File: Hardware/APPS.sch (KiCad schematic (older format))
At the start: 20 parts, among them SW1 SW_Push, U1 STM32F103C8Tx, Y1 Crystal 8 MHz

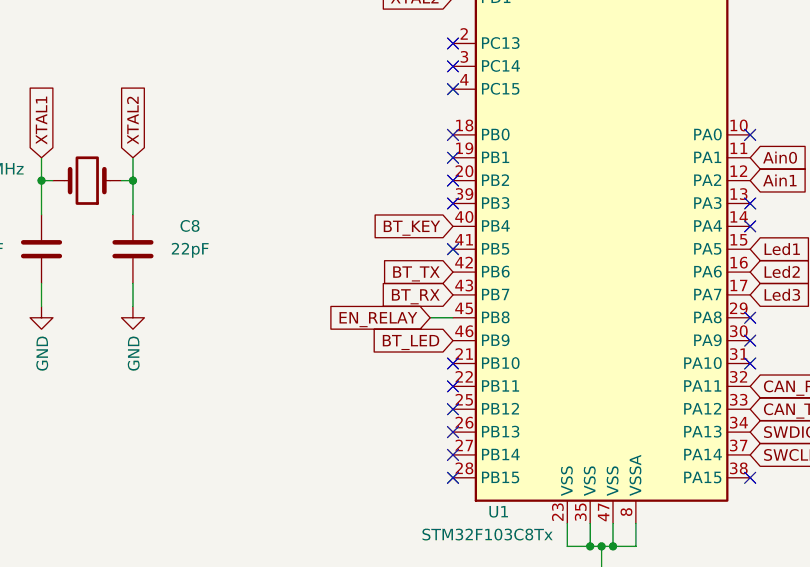
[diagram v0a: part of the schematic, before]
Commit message: Quick fixes
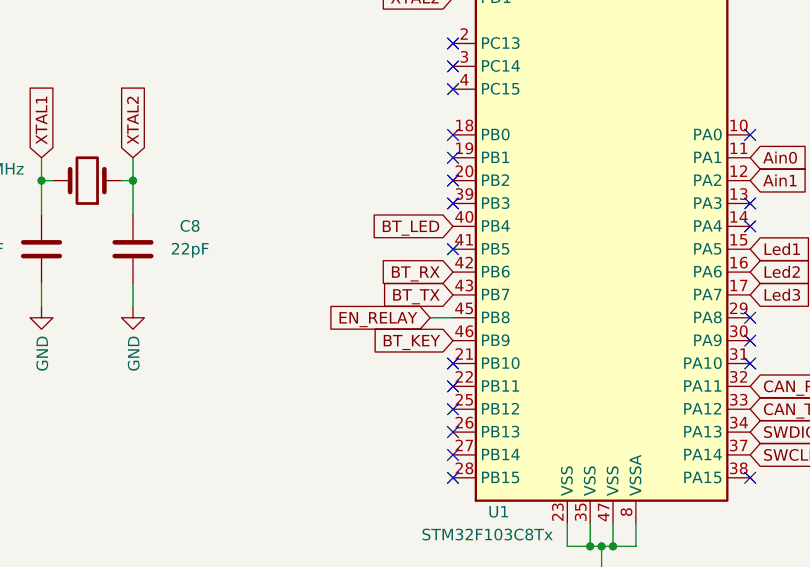
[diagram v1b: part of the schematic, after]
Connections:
- net BT_KEY: now also U1.46 (PB9); no longer U1.40 (PB4)
- net BT_LED: now also U1.40 (PB4); no longer U1.46 (PB9)
- net BT_RX: now also U1.42 (PB6); no longer U1.43 (PB7)
- net BT_TX: now also U1.43 (PB7); no longer U1.42 (PB6)
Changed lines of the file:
@@
 NoConn ~ 4200 4850
 NoConn ~ 4200 4750
-NoConn ~ 4200 4650
-NoConn ~ 4200 4150
 NoConn ~ 5500 4050
 NoConn ~ 5500 3950
@@
 Text Notes 7850 2700 0    50   ~ 0
 Debugging Diodes
-Text GLabel 4200 4350 0    50   Input ~ 0
-BT_RX
-Text GLabel 4200 4250 0    50   Input ~ 0
-BT_TX
 Text GLabel 5500 4150 2    50   Input ~ 0
 Led1
-Text GLabel 4200 4050 0    50   Input ~ 0
-BT_KEY
-Text GLabel 4200 4550 0    50   Input ~ 0
-BT_LED
 NoConn ~ 5500 4550
 NoConn ~ 5500 4650
 Text GLabel 5500 4750 2    50   Input ~ 0
 CAN_RX
+Text GLabel 4200 4550 0    50   Input ~ 0
+BT_KEY
+NoConn ~ 4200 4650
+Text GLabel 4200 4250 0    50   Input ~ 0
+BT_RX
+Text GLabel 4200 4350 0    50   Input ~ 0
+BT_TX
+NoConn ~ 4200 4150
+Text GLabel 4200 4050 0    50   Input ~ 0
+BT_LED
 $EndSCHEMATC
